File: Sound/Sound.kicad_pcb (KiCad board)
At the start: 2 copper layers, 100 x 100 mm, 58 parts, among them J1 Buss, SW1 Slot, U1 YM2149, U2 74LS85, U3 74LS00, U4 SAA1099, U5 74LS139, U6 YM2149, U7 SAA1099, Y1 8MHz

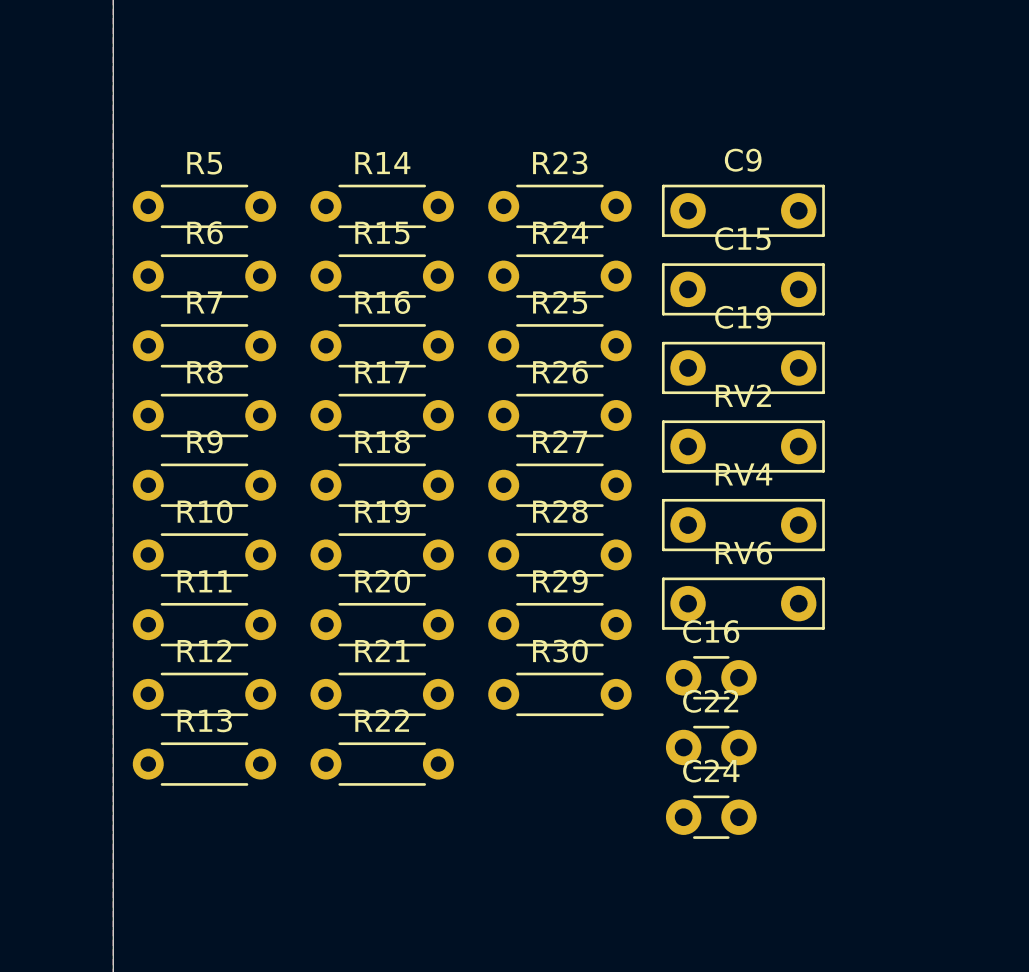
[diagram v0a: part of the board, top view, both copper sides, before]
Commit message: added galasm ref
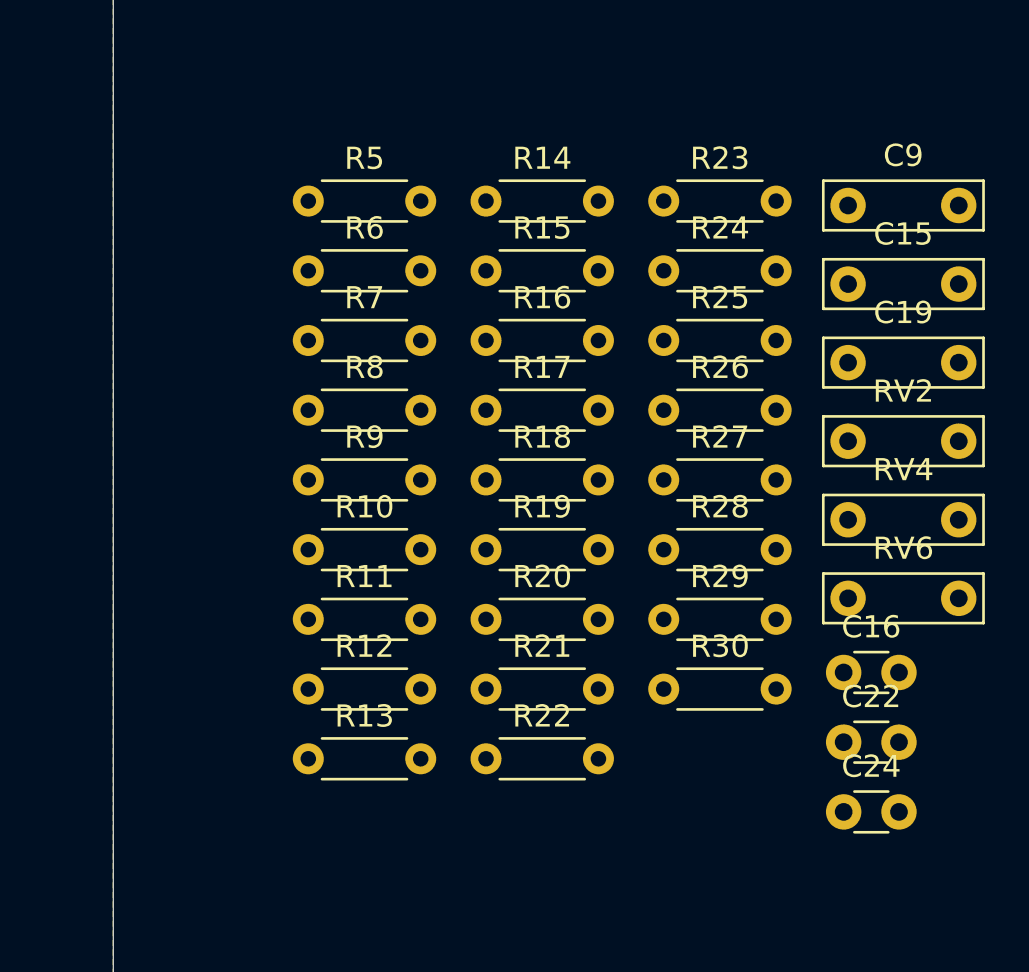
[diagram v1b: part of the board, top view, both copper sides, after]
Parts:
- moved R23 7.23 mm to (149.9, 53.0)
- moved R24 7.23 mm to (149.9, 56.2)
- moved R25 7.23 mm to (149.9, 59.3)
- moved R26 7.23 mm to (149.9, 62.5)
- moved R27 7.23 mm to (149.9, 65.6)
- moved R28 7.23 mm to (149.9, 68.8)
- moved R29 7.23 mm to (149.9, 71.9)
- moved R30 7.23 mm to (149.9, 75.1)
- moved R10 7.23 mm to (133.8, 68.8)
- moved R11 7.23 mm to (133.8, 71.9)
- moved R12 7.23 mm to (133.8, 75.1)
- moved R13 7.23 mm to (133.8, 78.2)
- moved R5 7.23 mm to (133.8, 53.0)
- moved R6 7.23 mm to (133.8, 56.2)
- moved R7 7.23 mm to (133.8, 59.3)
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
